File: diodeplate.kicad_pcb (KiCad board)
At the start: 2 copper layers, 86 parts, among them U1 TS-1185EC-C-D-B, U10 CP2102-GMR, U11 U262-16XN-4BVC11, U14 UMH3N, U2 TS-1185EC-C-D-B, U3 TS-1185EC-C-D-B, U8 ESP32-WROOM-32E(4MB), U9 SN74AHCT32QPWRQ1

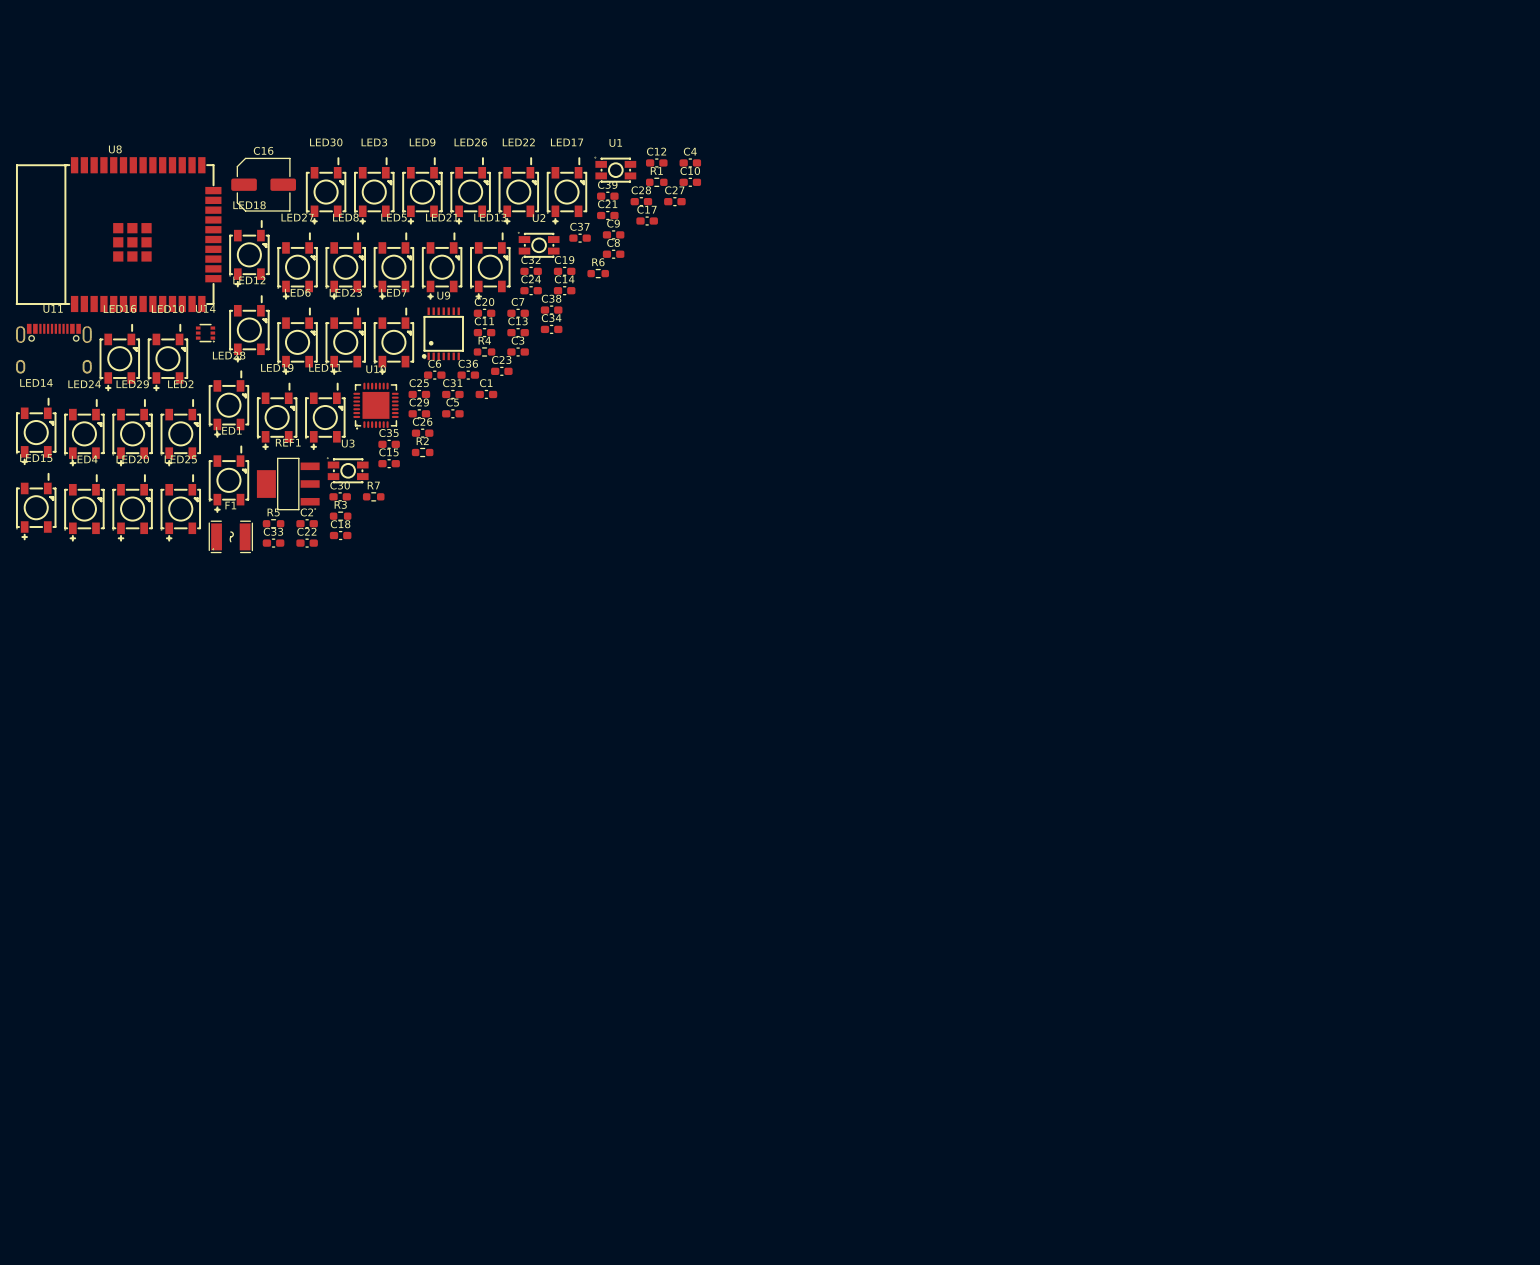
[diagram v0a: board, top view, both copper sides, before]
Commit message: add first pcb design
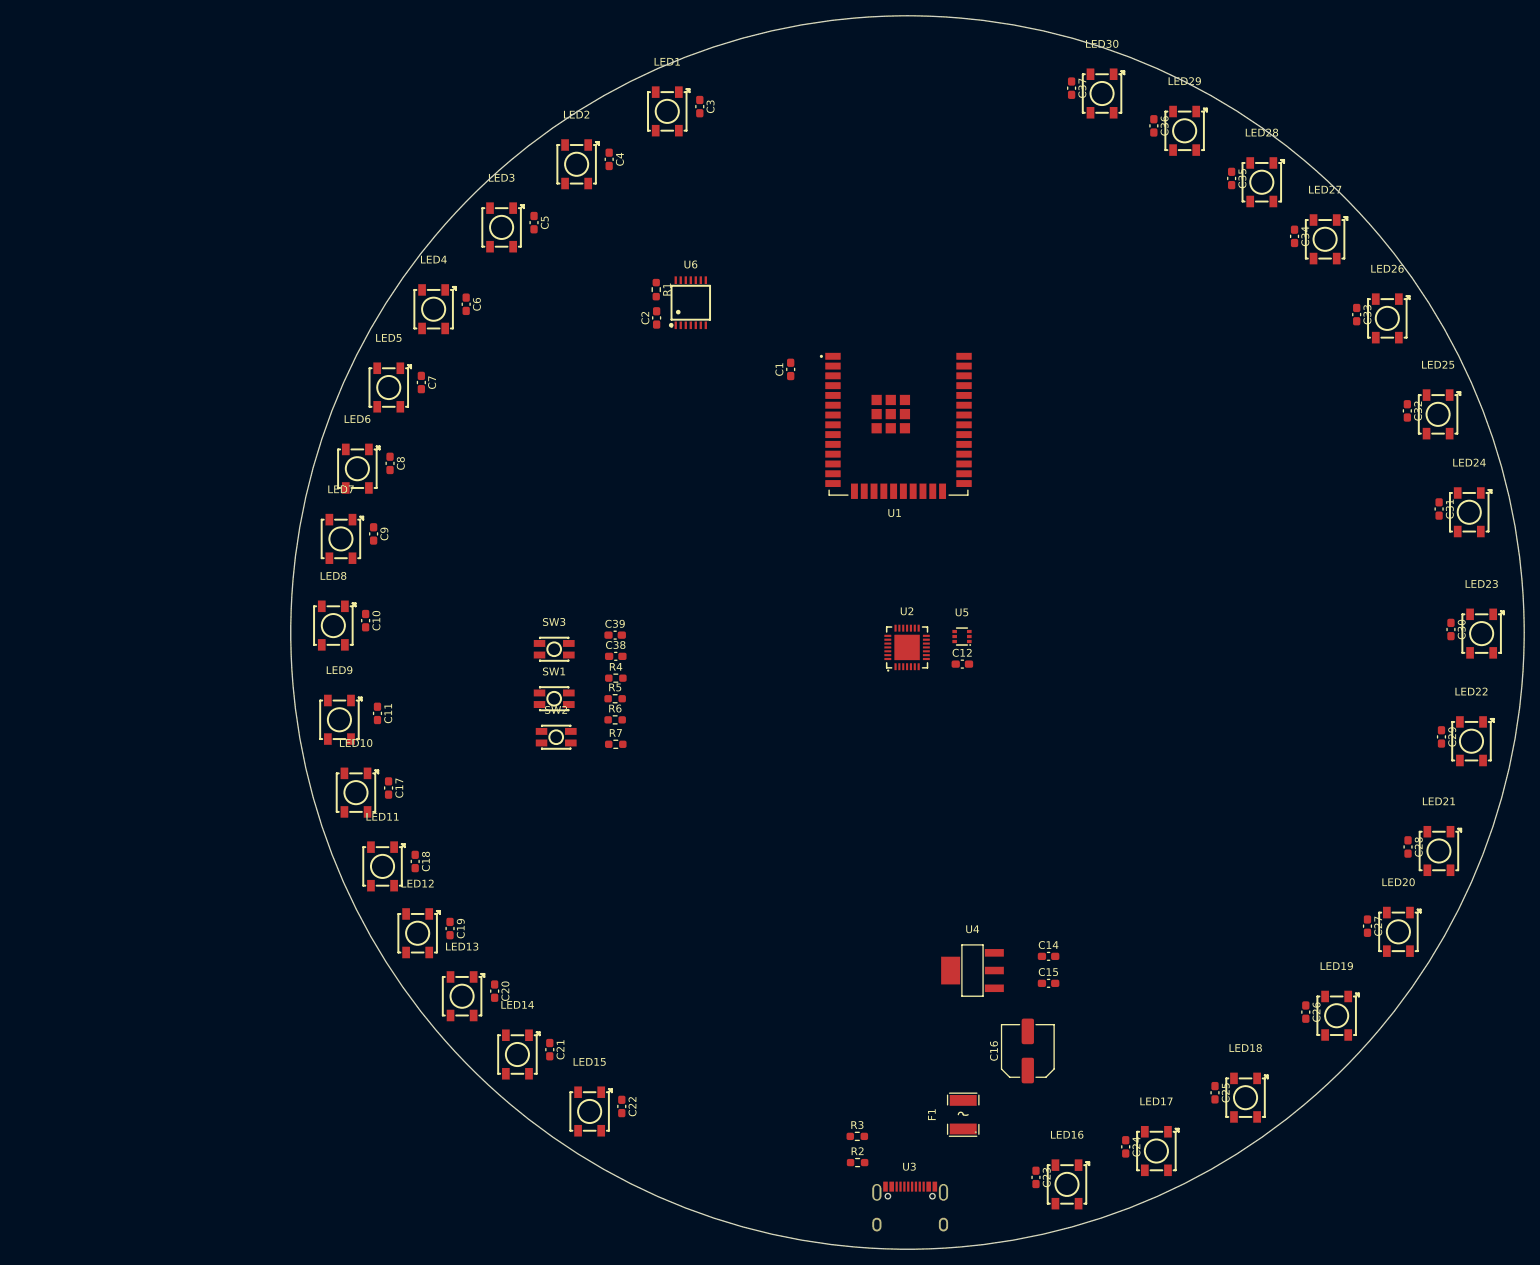
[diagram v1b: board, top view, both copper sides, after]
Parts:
- removed C13: 10uF, Capacitor_SMD:C_0603_1608Metric_Pad1.08x0.95mm_HandSolder
- removed REF1: BL1117-33CX, footprint:SOT-223-4_L6.5-W3.5-P2.30-LS7.0-BR
- removed U10: CP2102-GMR, footprint:QFN-28_L5.0-W5.0-P0.50-BL-EP
- removed U11: U262-16XN-4BVC11, footprint:USB-3.1-SMD_U262-161N-4BVC11
- removed U14: UMH3N, footprint:SC-70-6_L2.2-W1.3-P0.65-LS2.1-BR
- removed U8: ESP32-WROOM-32E(4MB), footprint:WIFI-SMD_ESP32-WROOM-32E
- removed U9: SN74AHCT32QPWRQ1, footprint:TSSOP-14_L5.0-W4.4-P0.65-LS6.5-BL
- added SW1: TS-1185EC-C-D-B, footprint:SW-SMD_4P-L3.7-W3.0-P1.50-LS4.7, F.Cu at (170.8, 151.2)
- added SW2: TS-1185EC-C-D-B, footprint:SW-SMD_4P-L3.7-W3.0-P1.50-LS4.7, F.Cu at (171.0, 156.2)
- added SW3: TS-1185EC-C-D-B, footprint:SW-SMD_4P-L3.7-W3.0-P1.50-LS4.7, F.Cu at (170.8, 144.8)
- added U4: BL1117-33CX, footprint:SOT-223-4_L6.5-W3.5-P2.30-LS7.0-BR, F.Cu at (225.0, 186.5)
- added U5: UMH3N, footprint:SC-70-6_L2.2-W1.3-P0.65-LS2.1-BR, F.Cu at (223.7, 143.1)
- added U6: SN74AHCT32QPWRQ1, footprint:TSSOP-14_L5.0-W4.4-P0.65-LS6.5-BL, F.Cu at (188.5, 99.8)
- U1: value TS-1185EC-C-D-B -> ESP32-WROOM-32E; footprint footprint:SW-SMD_4P-L3.7-W3.0-P1.50-LS4.7 -> footprint:WIFI-SMD_ESP32-WROOM-32E
- U2: value TS-1185EC-C-D-B -> CP2102-GMR; footprint footprint:SW-SMD_4P-L3.7-W3.0-P1.50-LS4.7 -> footprint:QFN-28_L5.0-W5.0-P0.50-BL-EP
- U3: value TS-1185EC-C-D-B -> U262-161N-4BVC11; footprint footprint:SW-SMD_4P-L3.7-W3.0-P1.50-LS4.7 -> footprint:USB-3.1-SMD_U262-161N-4BVC11
- moved LED24 179.9 mm to (289.5, 126.9)
- moved LED20 173.1 mm to (280.3, 181.3)
- moved LED18 169.3 mm to (260.5, 202.8)
- moved LED25 163.6 mm to (285.4, 114.2)
- moved LED16 163.0 mm to (237.3, 214.1)
- moved LED19 157.8 mm to (272.3, 192.2)
- moved LED23 152.1 mm to (291.1, 142.6)
- moved LED21 149.9 mm to (285.5, 170.8)
- moved C16 149.8 mm to (232.2, 196.9), turned to 90 degrees
- moved LED17 146.0 mm to (248.9, 209.7)
- moved C30 145.1 mm to (287.1, 142.2), turned to -90 degrees
- moved C33 143.6 mm to (274.9, 101.4), turned to -90 degrees
- moved LED22 142.6 mm to (289.8, 156.6)
- moved LED29 142.0 mm to (252.6, 77.4)
- moved C29 139.1 mm to (285.9, 156.2), turned to -90 degrees
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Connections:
- C1 pad 1: GND -> +3V3
- C1 pad 2: +3V3 -> GND
- U1 pad 2: Net-(R4-Pad1) -> +3V3
- U2 pad 1: GND -> unconnected-(U2-Pad1)
- U2 pad 2: Net-(R5-Pad1) -> unconnected-(U2-Pad2)
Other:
- board outline added: 160 x 160 mm
